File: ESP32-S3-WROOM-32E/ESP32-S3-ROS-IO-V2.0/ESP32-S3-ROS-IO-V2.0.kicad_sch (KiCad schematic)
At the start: 51 parts, among them J1 Conn_01x22_Socket, J10 XT30UPB-F, J11 XT30UPB-F, J12 XT30UPB-F, J13 XT30UPB-F, J14 XT30UPB-F, J15 XT30UPB-F, J16 XT60-M, J17 XT60-M, J2 Conn_01x22_Socket, J3 Conn_01x22_Socket, J4 Conn_01x22_Socket, J5 Conn_01x02_Pin, J8 XT30UPB-F, J9 XT30UPB-F, SW1 SW1, SW2 SW2, SW3 SW3, SW4 SW4, SW5 SW5, SW6 SW6, SW7 SW7, SW8 SW8, SW9 SW9

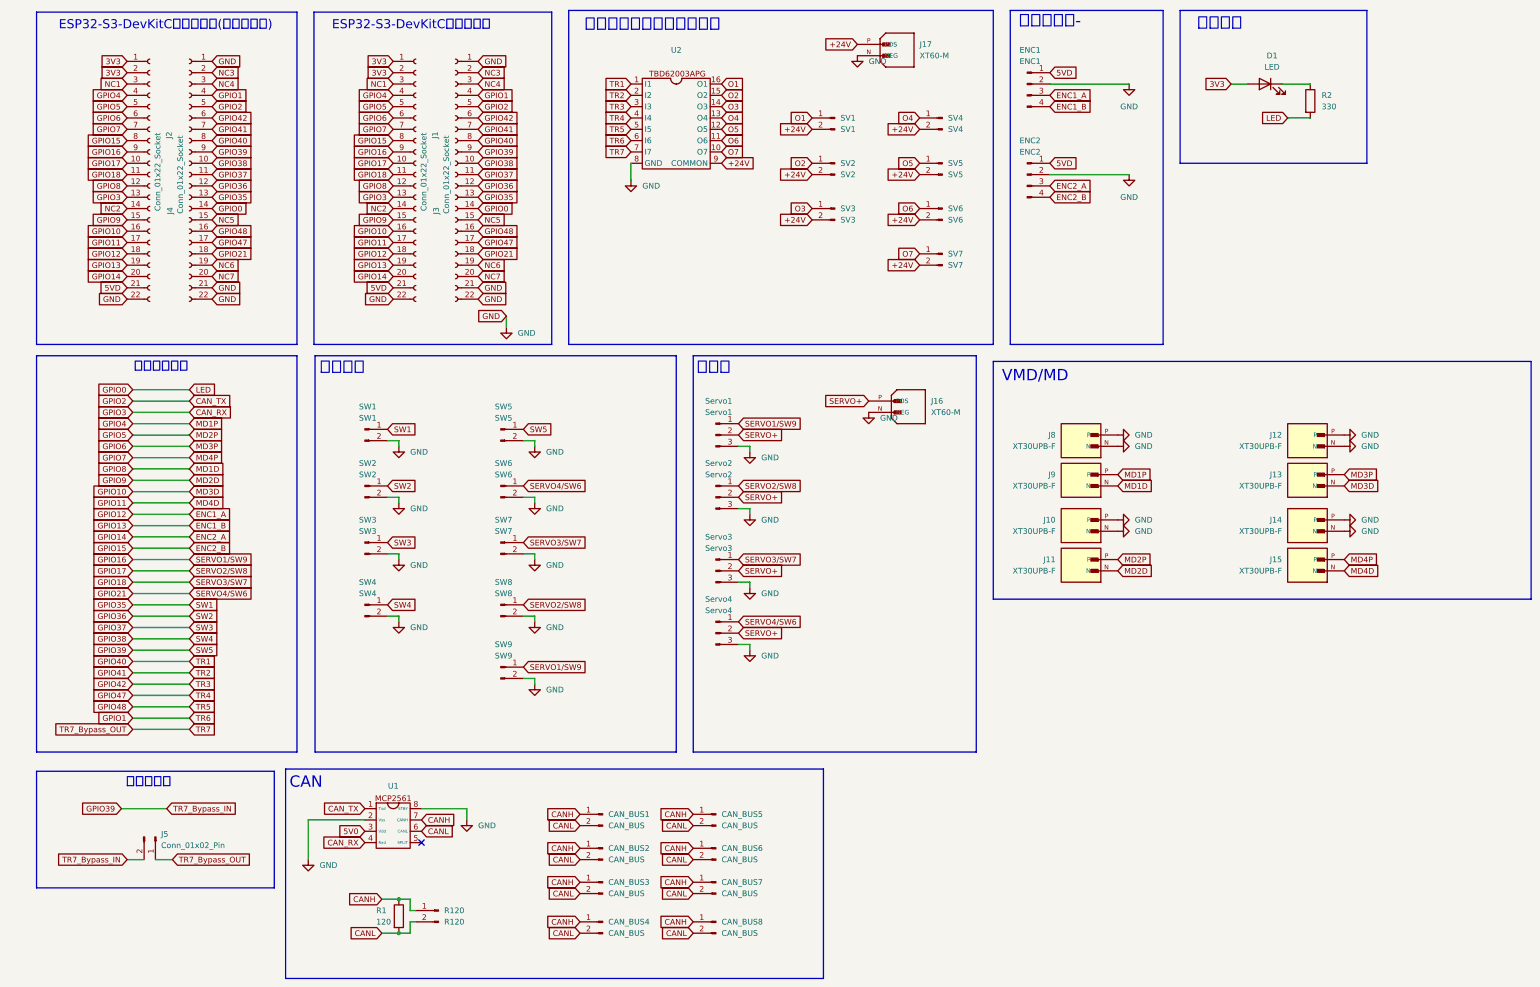
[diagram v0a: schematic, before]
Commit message: 新MD配置
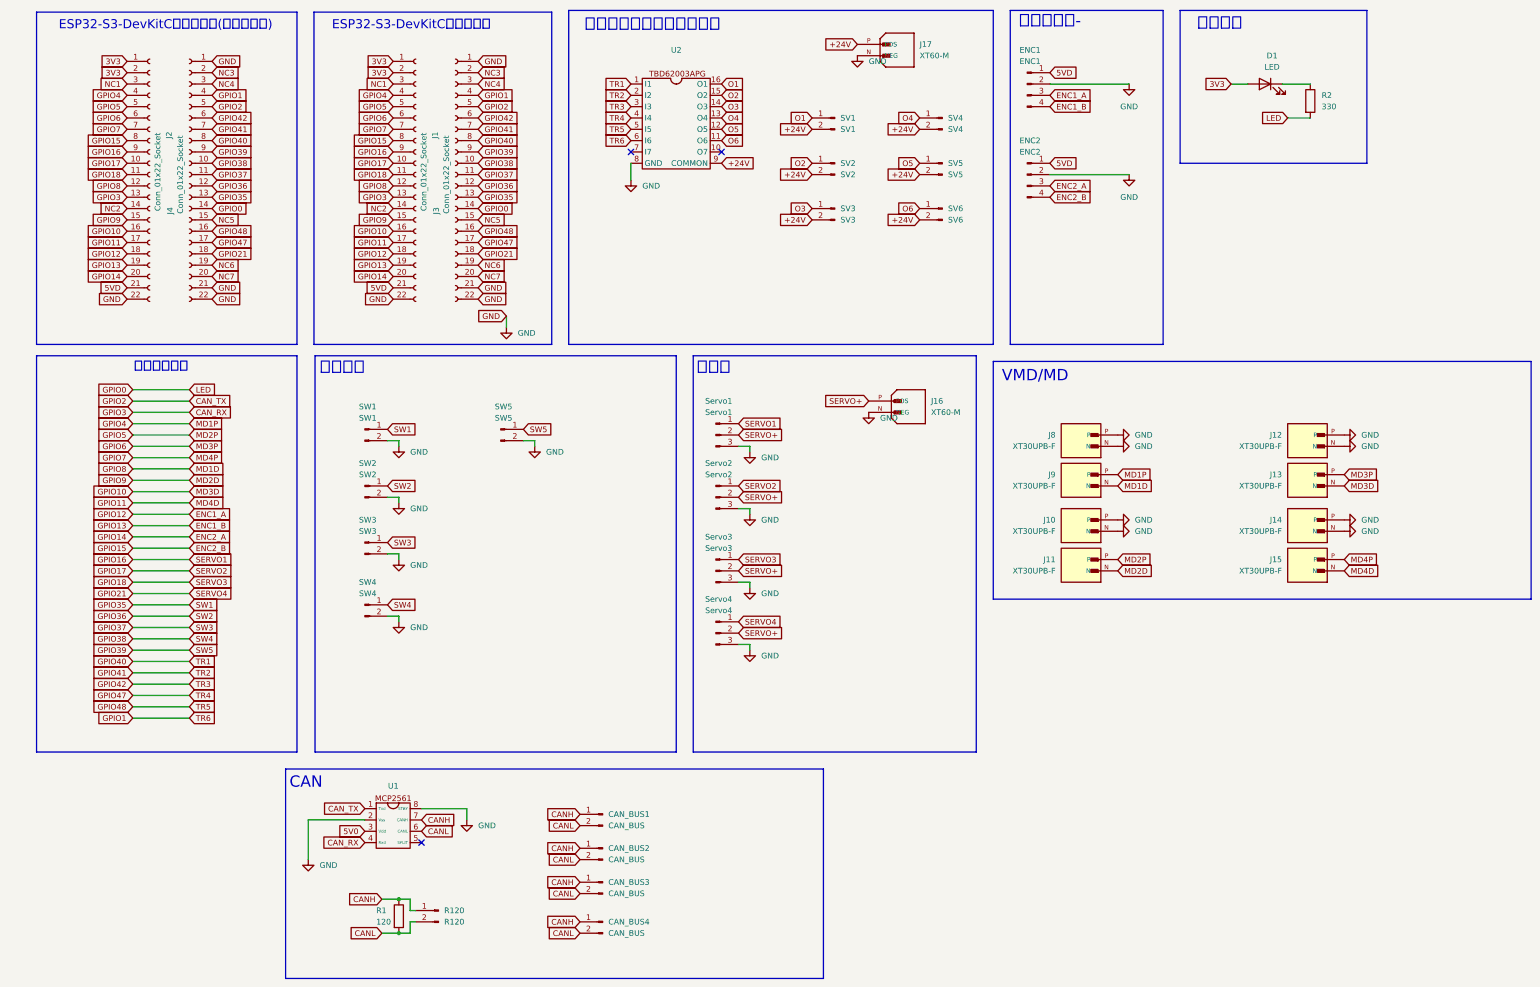
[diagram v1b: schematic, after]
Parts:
- removed CAN_BUS5, CAN_BUS6, CAN_BUS7, CAN_BUS8: CAN_BUS, Connector_JST:JST_XH_B2B-XH-A_1x02_P2.50mm_Vertical, symbol Connector:Conn_01x02_Pin
- removed J5: Conn_01x02_Pin, Connector_PinHeader_2.54mm:PinHeader_1x02_P2.54mm_Vertical, symbol Connector:Conn_01x02_Pin
- removed SV7: SV7, Connector_JST:JST_XH_B2B-XH-A_1x02_P2.50mm_Vertical, symbol Connector:Conn_01x02_Pin
- removed SW6: SW6, Connector_JST:JST_XH_B2B-XH-A_1x02_P2.50mm_Vertical, symbol Connector:Conn_01x02_Pin
- removed SW7: SW7, Connector_JST:JST_XH_B2B-XH-A_1x02_P2.50mm_Vertical, symbol Connector:Conn_01x02_Pin
- removed SW8: SW8, Connector_JST:JST_XH_B2B-XH-A_1x02_P2.50mm_Vertical, symbol Connector:Conn_01x02_Pin
- removed SW9: SW9, Connector_JST:JST_XH_B2B-XH-A_1x02_P2.50mm_Vertical, symbol Connector:Conn_01x02_Pin
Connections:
- net O7: no longer names the net of U2.10 (O7)
- net TR7: no longer names the net of U2.7 (I7)
- no-connect marks 1 -> 3
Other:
- note removed: "バイパス用"
